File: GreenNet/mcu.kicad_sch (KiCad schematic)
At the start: 11 parts, among them Q1 NPN, Q2 NPN, SW1 SW_Push, SW2 SW_Push, U1 ESP32-S3-WROOM-1-N16R2

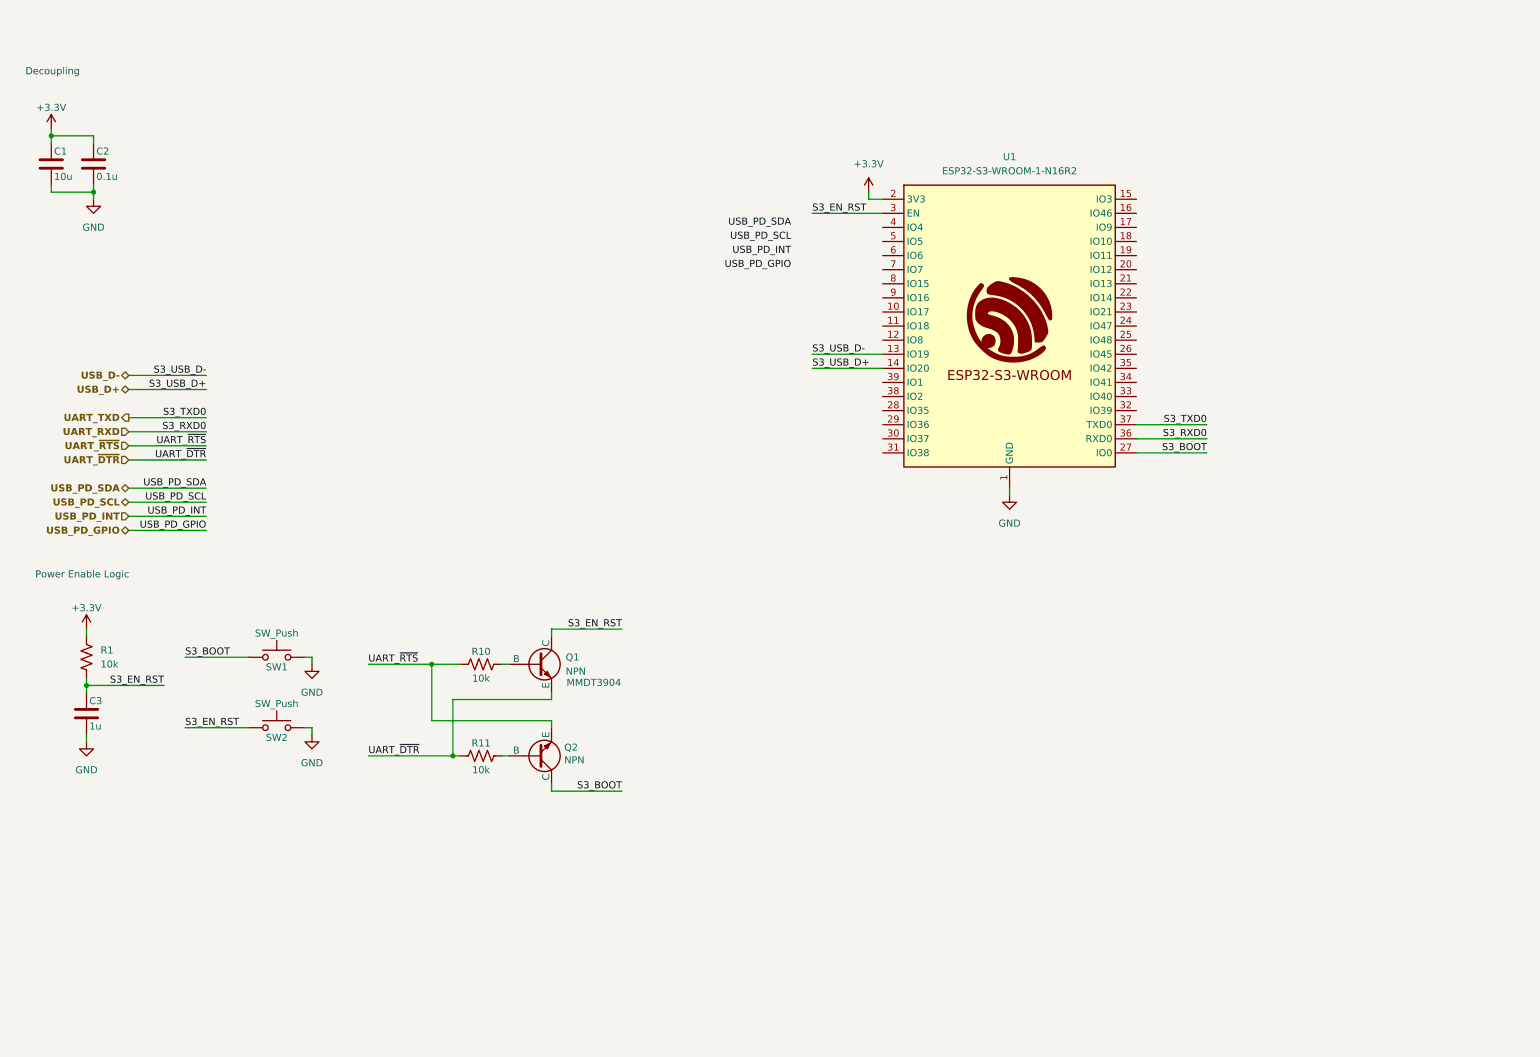
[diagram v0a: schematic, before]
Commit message: significant progress
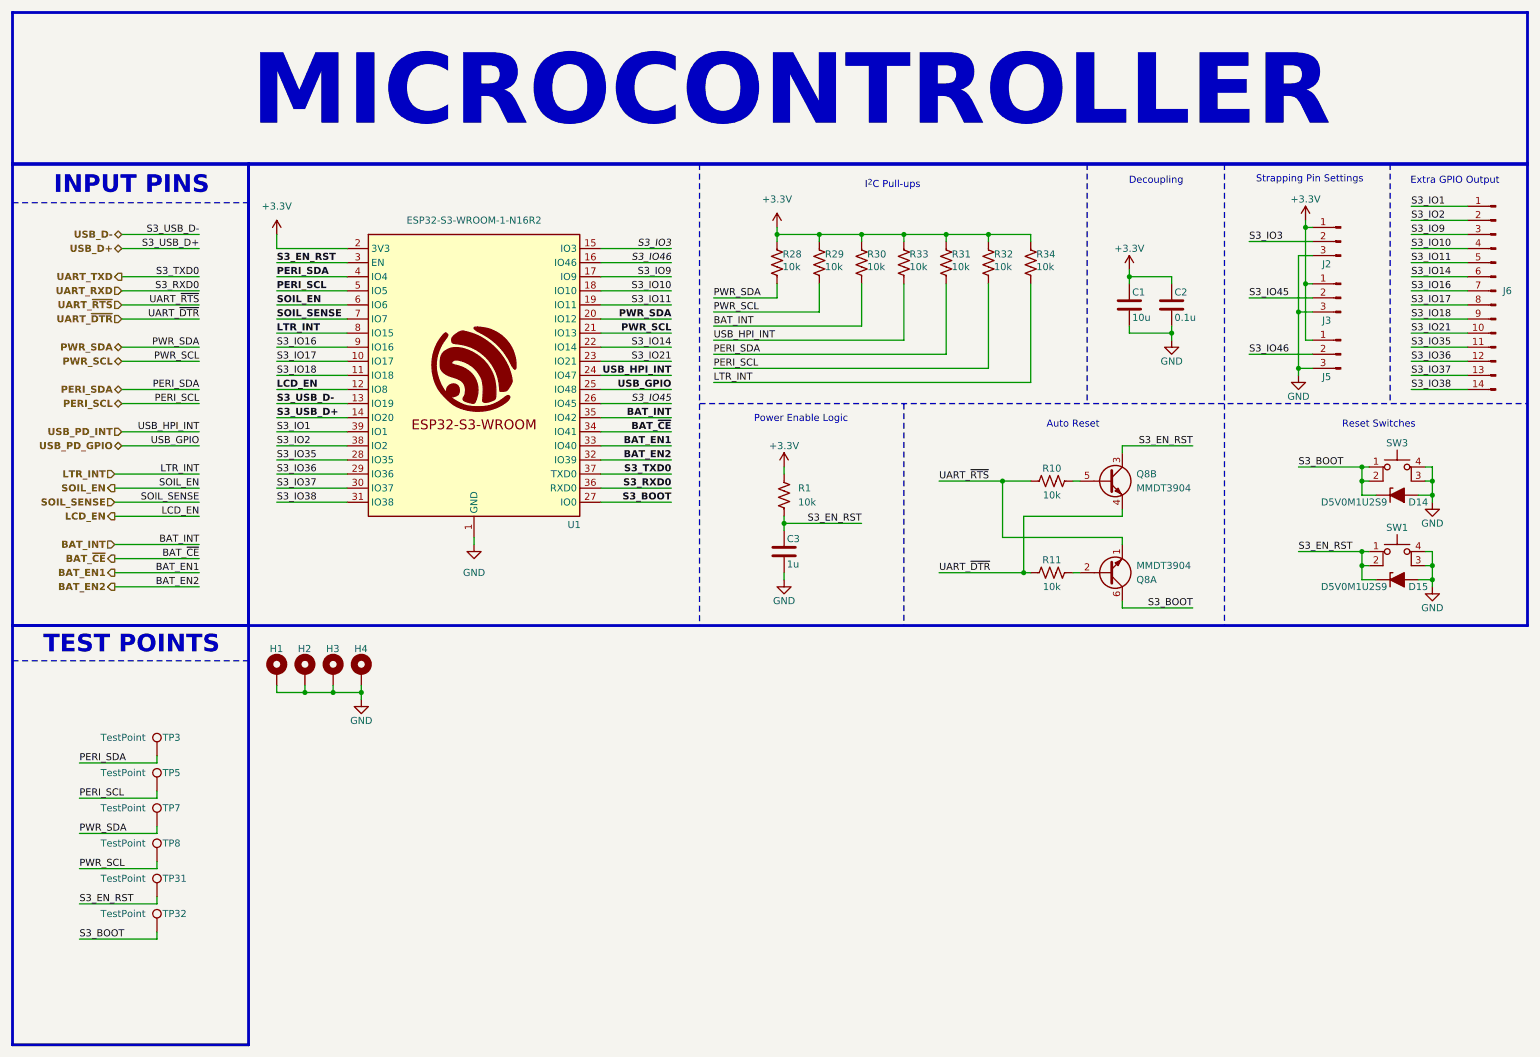
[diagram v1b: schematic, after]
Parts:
- removed Q1, Q2: NPN, symbol Simulation_SPICE:NPN
- removed SW1, SW2: SW_Push, symbol Switch:SW_Push
- added D14, D15: D5V0M1U2S9, AA_Diodes:D5V0M1U2S9Q, symbol Device:D_Zener_Filled
- added H1, H2, H3, H4: MountingHole_Pad, MountingHole:MountingHole_2.5mm_Pad, symbol Mechanical:MountingHole_Pad
- added J2, J3, J5: 3_Pin_Conn, AA_Connectors:61300311121, symbol Connector:Conn_01x03_Pin
- added J6: Conn_01x14_Pin, AA_Connectors:CONN_PH1-14-UA_ADM, symbol Connector:Conn_01x14_Pin
- added Q8: MMDT3904, Package_TO_SOT_SMD:SOT-363_SC-70-6, symbol Transistor_BJT:MMDT3904
- added R28, R29, R30, R31, R32, R33, R34: 10k, Resistor_SMD:R_0805_2012Metric, symbol Device:R_US
- added SW1, SW3: SW_MEC_5E, AA_Switches:18259106, symbol Switch:SW_MEC_5E
- added TP3, TP31, TP32, TP5, TP7, TP8: TestPoint, AA_TestPoints:RCWCTE, symbol Connector:TestPoint
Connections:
- net +3.3V: now also J2.1 (Pin_1), J3.1 (Pin_1), J5.1 (Pin_1), R28.2, R29.2, R30.2, R31.2, R32.2, R33.2, R34.2
- net EPAD: now also D14.2 (A), D15.2 (A), H1.1, H2.1, H3.1, H4.1, J2.3 (Pin_3), J3.3 (Pin_3), J5.3 (Pin_3), SW1.3 (K), SW1.4 (A), SW3.3 (K), SW3.4 (A)
- net S3_BOOT: now also D14.1 (K), Q8.6 (C1), SW3.1, SW3.2, TP32.1
- net S3_EN_RST: now also D15.1 (K), Q8.3 (C2), SW1.1, SW1.2, TP31.1
- net UART_~{DTR}: now also Q8.4 (E2)
- net UART_~{RTS}: now also Q8.1 (E1)
- net USB_PD_GPIO: now also U1.25 (IO48)
- net USB_PD_INT: now also U1.24 (IO47), R33.1
- net S3_IO17: now reaches U1.10 (IO17)
- net S3_IO17: now also J6.8 (Pin_8)
- net S3_IO18: now reaches U1.11 (IO18)
- net S3_IO18: now also J6.9 (Pin_9)
- net LCD_EN: now reaches U1.12 (IO8)
- net S3_IO3: now reaches U1.15 (IO3)
- net S3_IO3: now also J2.2 (Pin_2)
- net S3_IO46: now reaches U1.16 (IO46)
- net S3_IO46: now also J5.2 (Pin_2)
- net S3_IO9: now reaches U1.17 (IO9)
- net S3_IO9: now also J6.3 (Pin_3)
- net S3_IO10: now reaches U1.18 (IO10)
- net S3_IO10: now also J6.4 (Pin_4)
- net S3_IO11: now reaches U1.19 (IO11)
- net S3_IO11: now also J6.5 (Pin_5)
- net PWR_SDA: now reaches U1.20 (IO12)
- net PWR_SDA: now also R28.1, TP7.1
- net PWR_SCL: now reaches U1.21 (IO13)
- net PWR_SCL: now also R29.1, TP8.1
- net S3_IO14: now reaches U1.22 (IO14)
- net S3_IO14: now also J6.6 (Pin_6)
- net S3_IO21: now reaches U1.23 (IO21)
- net S3_IO21: now also J6.10 (Pin_10)
- net S3_IO45: now reaches U1.26 (IO45)
- net S3_IO45: now also J3.2 (Pin_2)
- net S3_IO35: now reaches U1.28 (IO35)
- net S3_IO35: now also J6.11 (Pin_11)
- net S3_IO36: now reaches U1.29 (IO36)
- net S3_IO36: now also J6.12 (Pin_12)
- net S3_IO37: now reaches U1.30 (IO37)
- net S3_IO37: now also J6.13 (Pin_13)
- net S3_IO38: now reaches U1.31 (IO38)
- net S3_IO38: now also J6.14 (Pin_14)
- net BAT_EN2: now reaches U1.32 (IO39)
- net BAT_EN1: now reaches U1.33 (IO40)
- net BAT_~{CE}: now reaches U1.34 (IO41)
- net BAT_INT: now reaches U1.35 (IO42)
- net BAT_INT: now also R30.1
- net S3_IO2: now reaches U1.38 (IO2)
- net S3_IO2: now also J6.2 (Pin_2)
- net S3_IO1: now reaches U1.39 (IO1)
- net S3_IO1: now also J6.1 (Pin_1)
- net PERI_SDA: now reaches U1.4 (IO4)
- net PERI_SDA: now also R31.1, TP3.1
- net PERI_SCL: now reaches U1.5 (IO5)
- net PERI_SCL: now also R32.1, TP5.1
- net SOIL_EN: now reaches U1.6 (IO6)
- net SOIL_SENSE: now reaches U1.7 (IO7)
- net LTR_INT: now reaches U1.8 (IO15)
- net LTR_INT: now also R34.1
- net S3_IO16: now reaches U1.9 (IO16)
- net S3_IO16: now also J6.7 (Pin_7)
- net at R10.2: now also Q8.5 (B2)
- net at R11.2: now also Q8.2 (B1)
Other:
- note added: "Auto Reset"
- note added: "Extra GPIO Output"
- note added: "INPUT PINS"
- note added: "I^{2}C Pull-ups"
- note added: "MICROCONTROLLER"
- note added: "Reset Switches"
- note added: "Strapping Pin Settings"
- note added: "TEST POINTS"
- moved on the sheet: C1, C2, C3, R1, R10, R11, U1
